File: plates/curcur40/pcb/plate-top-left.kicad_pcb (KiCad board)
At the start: 2 copper layers, 116.1 x 88.3 mm, 0 parts

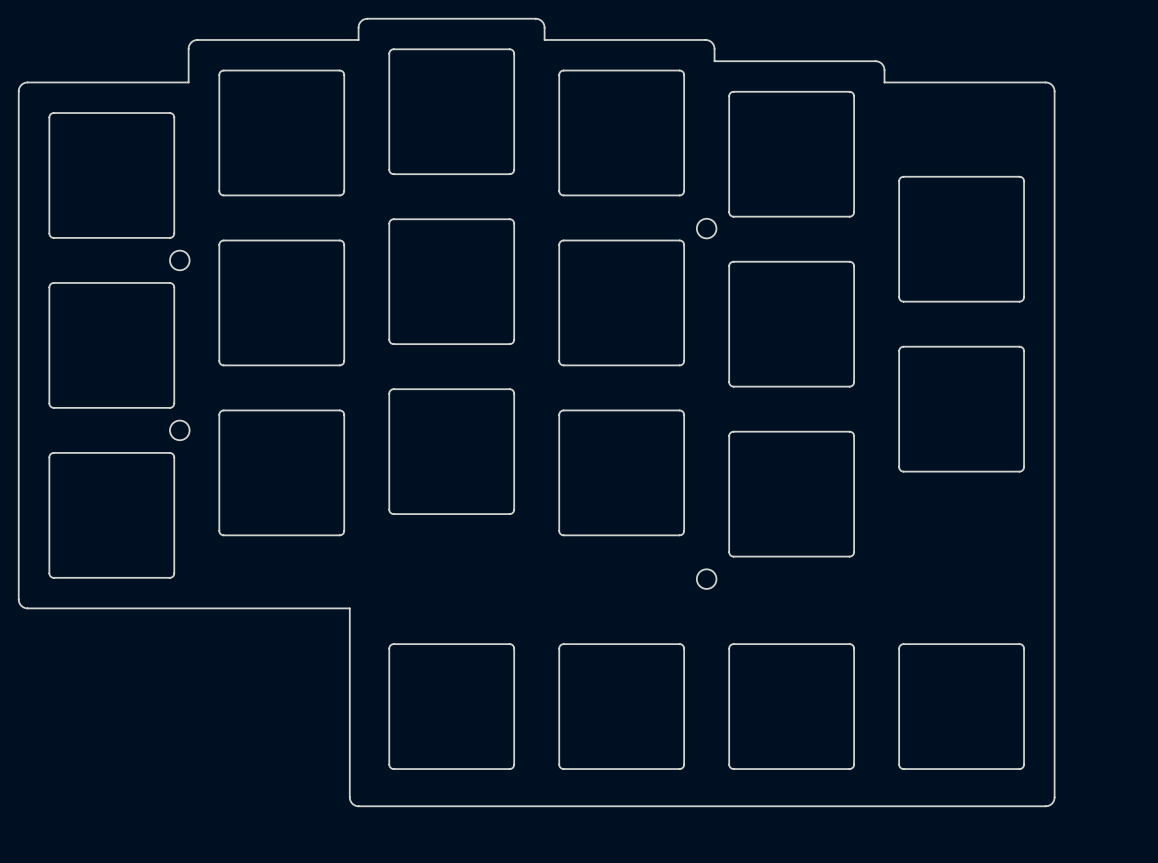
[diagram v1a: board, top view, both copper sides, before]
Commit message: fix all
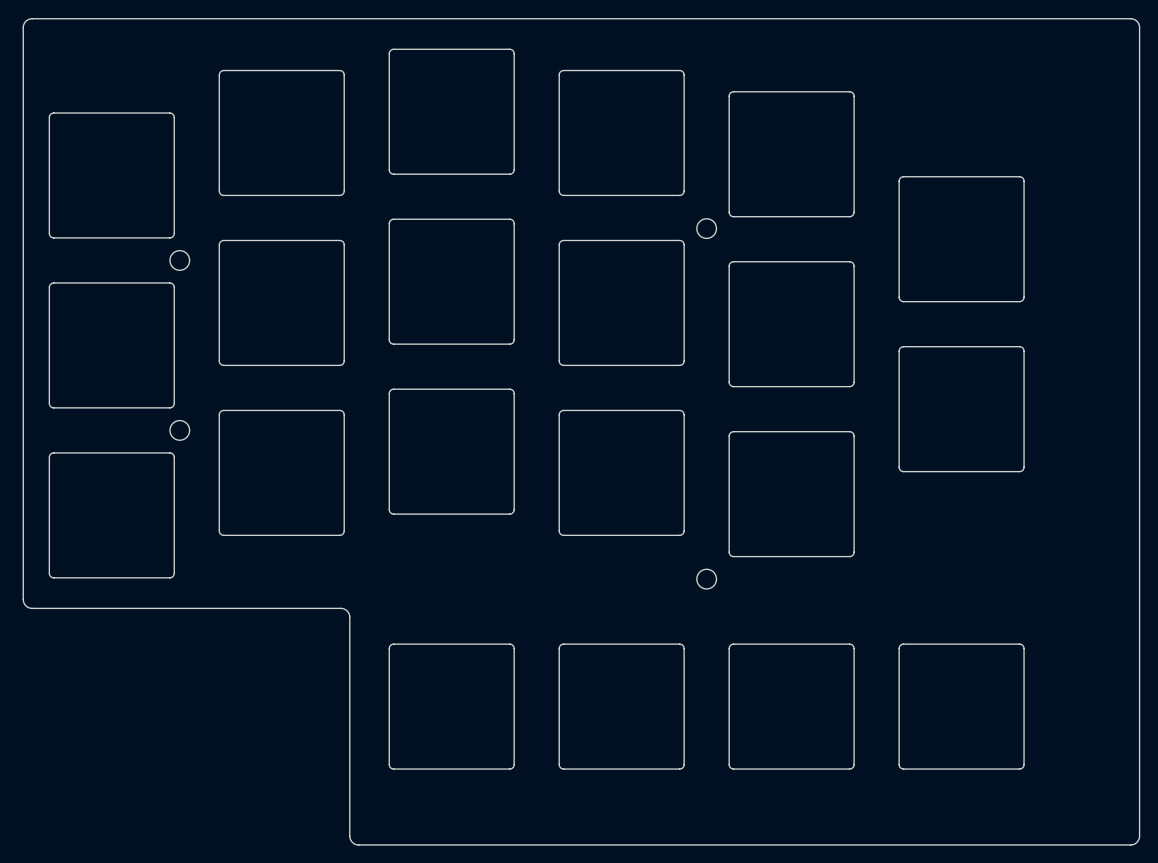
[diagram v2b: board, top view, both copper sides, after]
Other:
- board size 116.1 x 88.3 mm -> 125.1 x 92.6 mm
- rule pad_to_mask_clearance: 0.2 -> 0
